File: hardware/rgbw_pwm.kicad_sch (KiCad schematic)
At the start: 6 parts, among them J201 B5B-XH-A, J202 B5B-XH-A, Q201 DMN2041LSD, Q202 DMN2041LSD, Q203 DMN2041LSD, Q204 DMN2041LSD

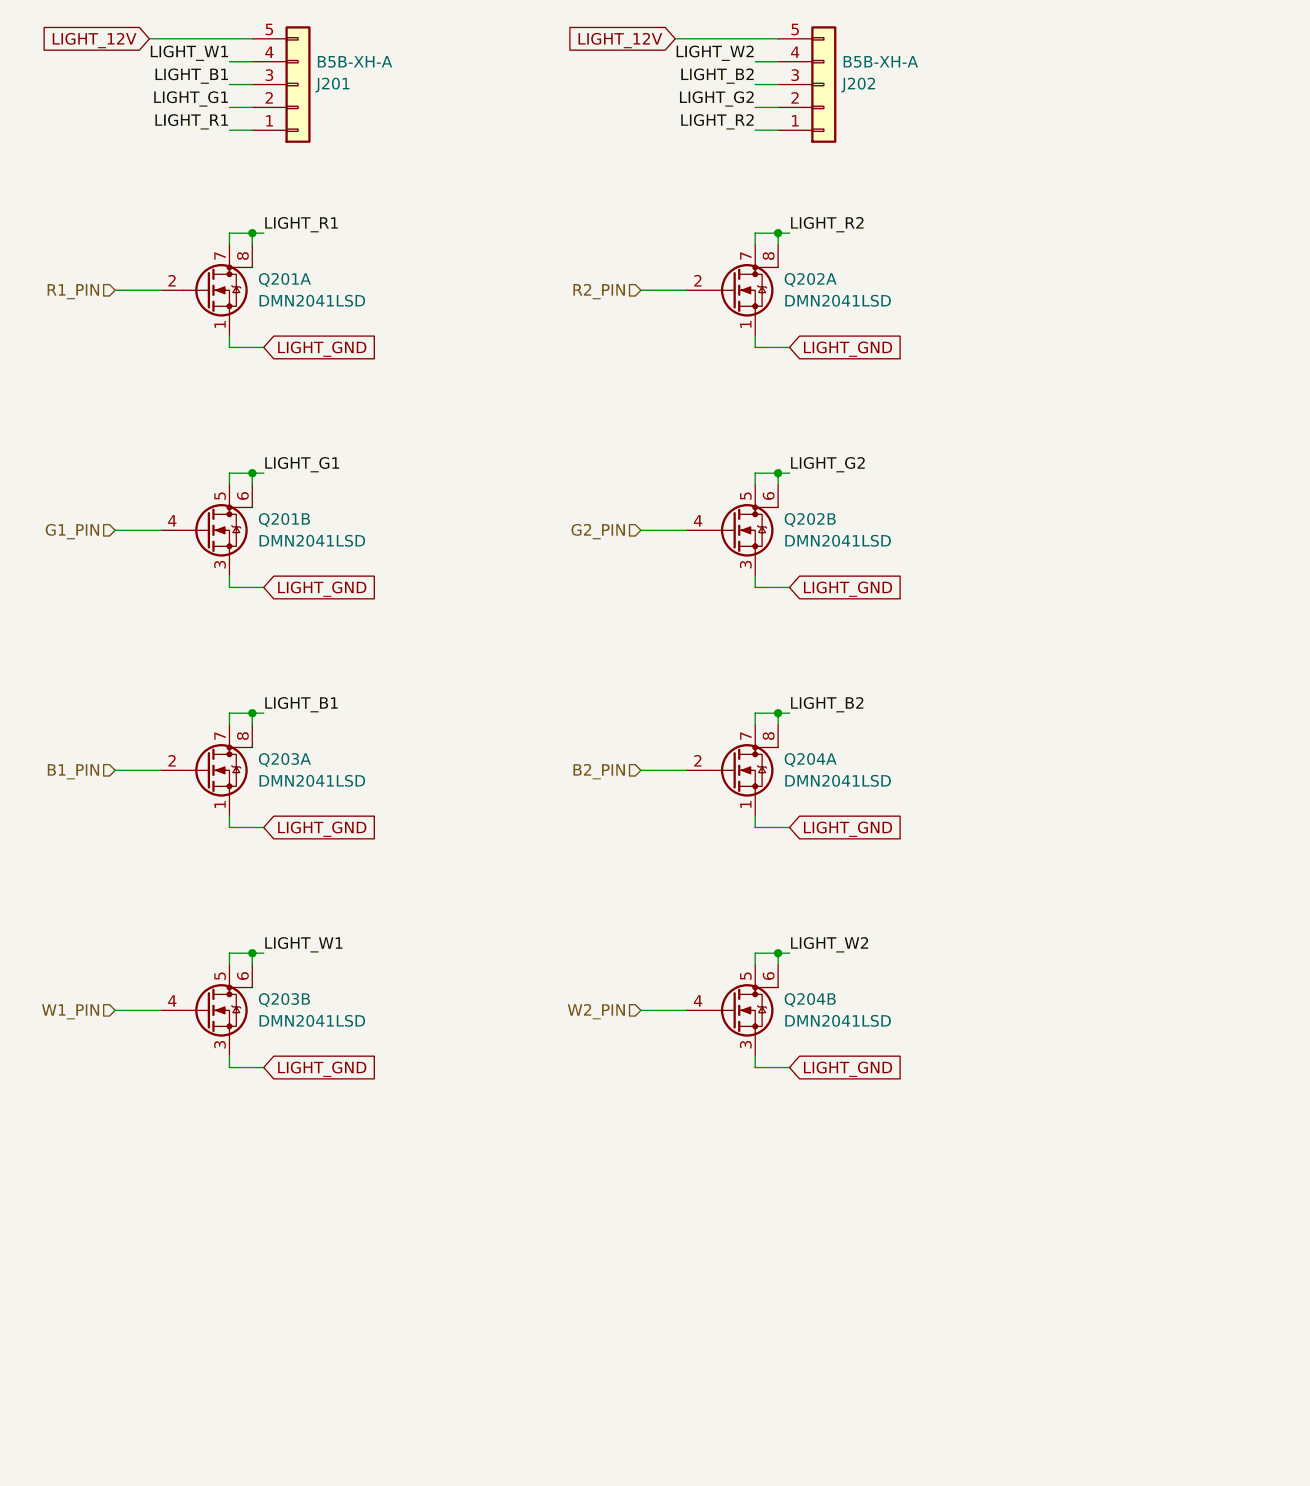
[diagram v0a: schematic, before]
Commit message: Tidy up the schematic.
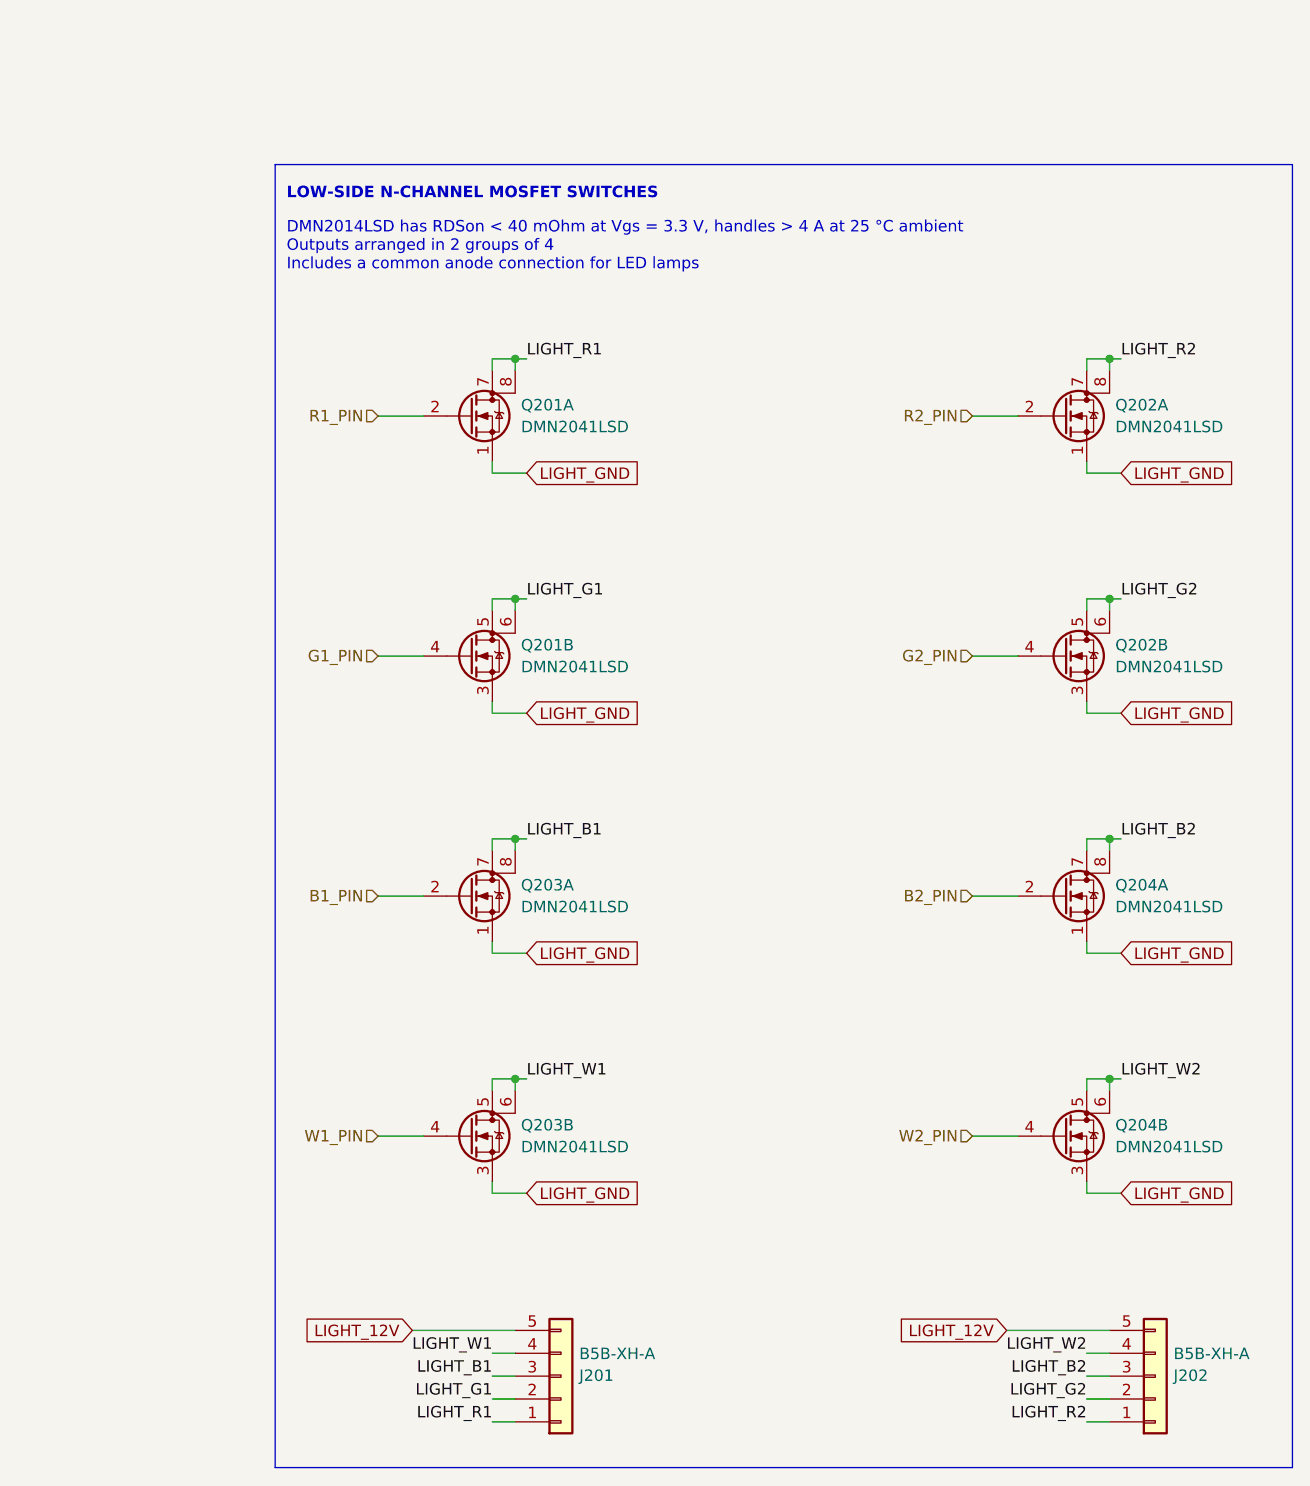
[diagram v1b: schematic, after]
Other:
- note added: "DMN2014LSD has RDSon < 40 mOhm at Vgs = 3.3 V, handles > 4 A at 25 °C ambient Outputs arranged in 2 groups of 4 Includes a common anode connection for LED lamps"
- note added: "LOW-SIDE N-CHANNEL MOSFET SWITCHES"
- moved on the sheet: J201, J202, Q201A, Q201B, Q202A, Q202B, Q203A, Q203B, Q204A, Q204B
